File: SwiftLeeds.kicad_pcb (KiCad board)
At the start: 2 copper layers, 54.3 x 74.6 mm, 13 parts

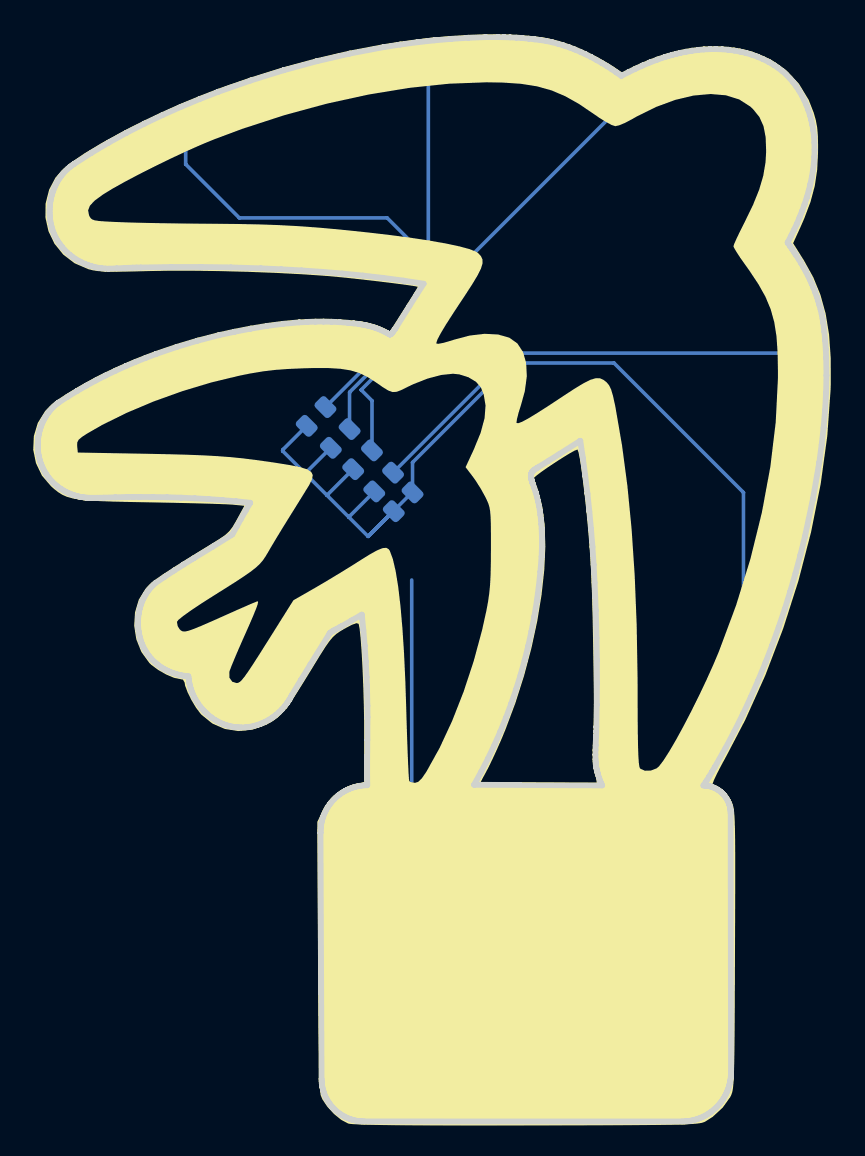
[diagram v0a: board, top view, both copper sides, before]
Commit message: V.... 5 I think? Idk anymore, time has become one long unending torture
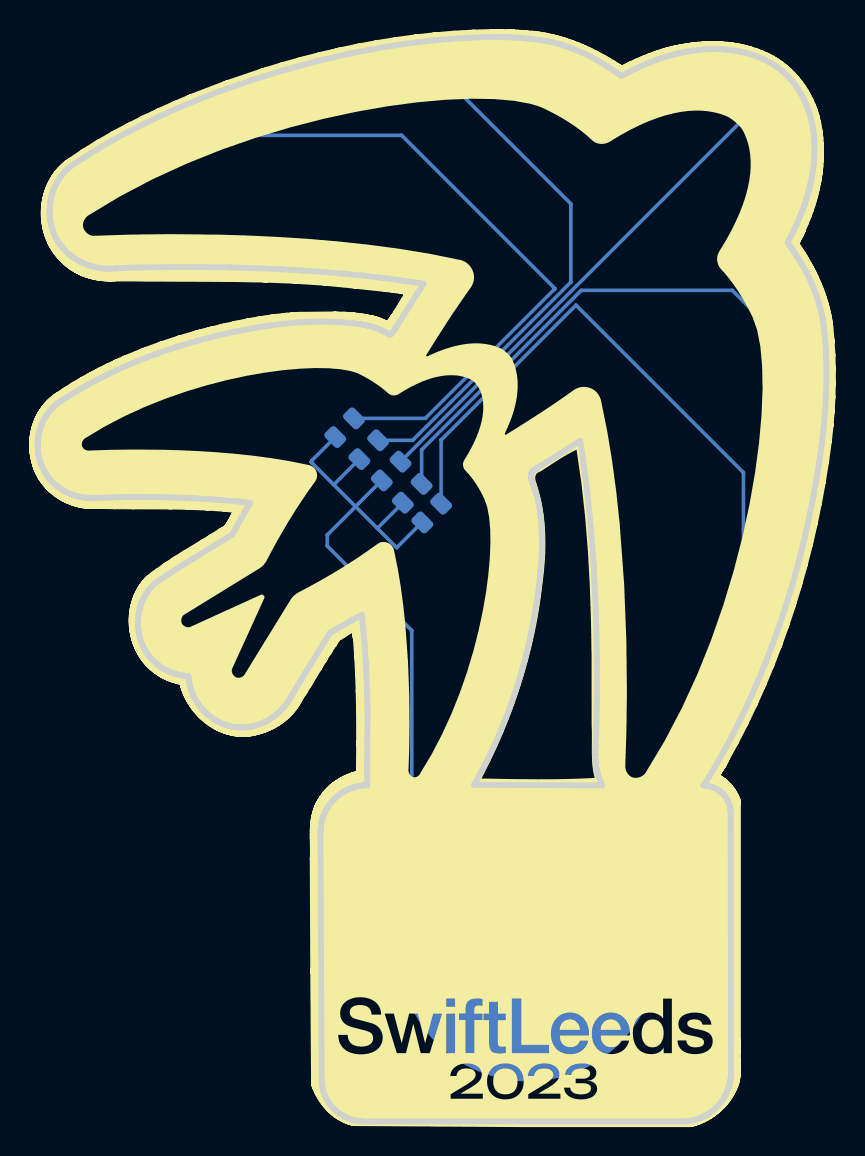
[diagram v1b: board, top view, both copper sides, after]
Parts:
- removed the G*** at (141.0, 78.0)
- D1, D2, D3, D4, D5: footprint LED_SMD:LED_0805_2012Metric -> LED_SMD:LED_0805_Side
- moved R2 2.11 mm to (136.6, 69.1)
- moved R3 2.11 mm to (138.2, 70.6)
- moved R4 2.11 mm to (139.6, 72.1)
- moved R5 2.11 mm to (141.0, 73.4)
- moved R1 2.11 mm to (135.0, 67.6)
- moved G*** 0.95 mm to (140.2, 78.9)
- turned BT2 to 0 degrees
- turned D1 to 25 degrees
- turned D2 to 0 degrees
- turned D3 to -45 degrees
- turned D4 to -90 degrees
- turned D5 to -110 degrees
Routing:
- net Net-(D1-Pad2): track 35.6 -> 47.5 mm
- net Net-(D2-Pad2): track 28.2 -> 36.8 mm
- net Net-(D3-Pad2): track 40.9 -> 36.1 mm
- net Net-(BT2-Pad1): track 79.4 -> 83.4 mm
- net Net-(D5-Pad2): track 41.8 -> 45.6 mm
- net Net-(D4-Pad2): track 31.0 -> 34.4 mm
- net Net-(BT2-Pad2): track 126.8 -> 124.1 mm

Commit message: lmao, what the fuck is wrong with me - version 7 lets goooo
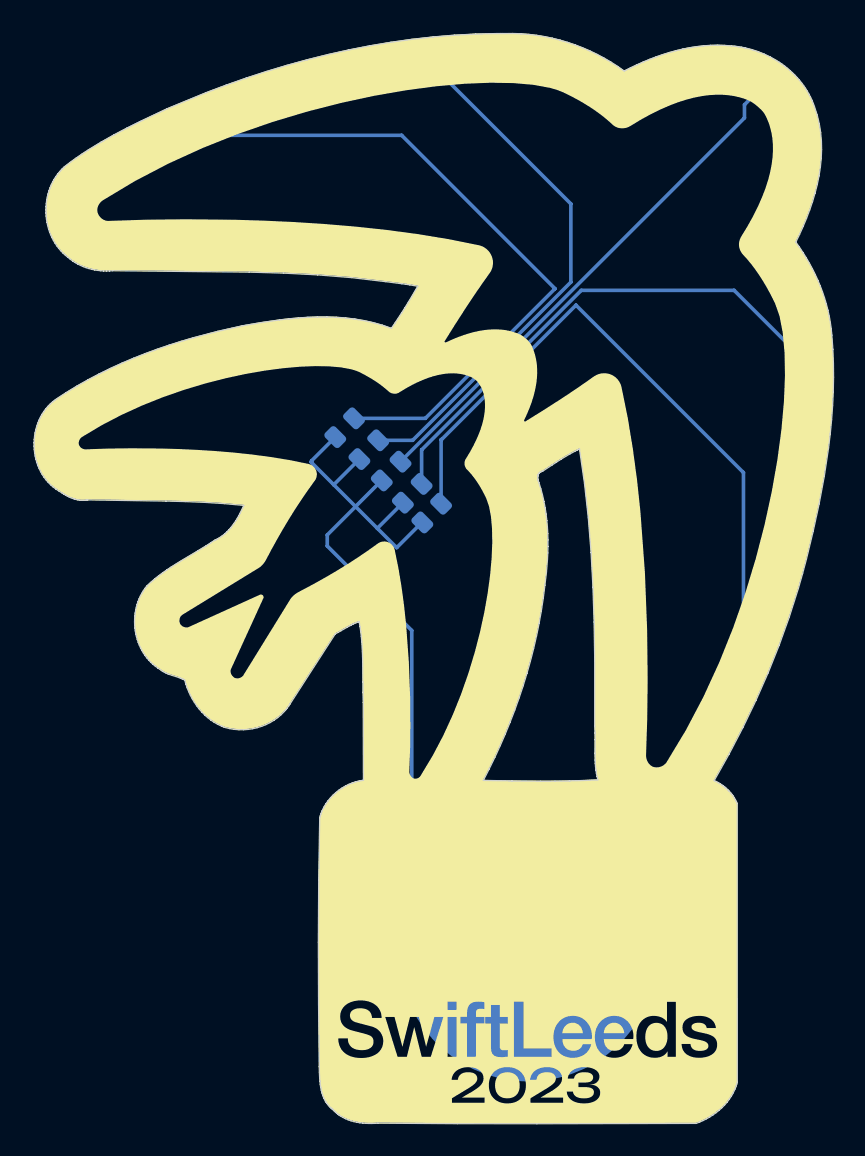
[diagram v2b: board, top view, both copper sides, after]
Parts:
- removed G***: LOGO, Birb:mask_big_birb
- moved D4 0.99 mm to (166.7, 64.0)
- moved D3 0.75 mm to (164.4, 44.7)
- moved D5 0.43 mm to (162.5, 83.5)
- turned D2 to 6 degrees
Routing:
- net Net-(BT2-Pad2): track 124.1 -> 127.3 mm
- net Net-(D4-Pad2): track 34.4 -> 35.4 mm
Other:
- board size 54.3 x 74.6 mm -> 55 x 75 mm
